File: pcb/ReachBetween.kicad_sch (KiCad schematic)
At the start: 7 parts, among them J1 USB_C_Receptacle_USB2.0, J2 USB_C_Receptacle_USB2.0, J3 USB_C_Receptacle_USB2.0

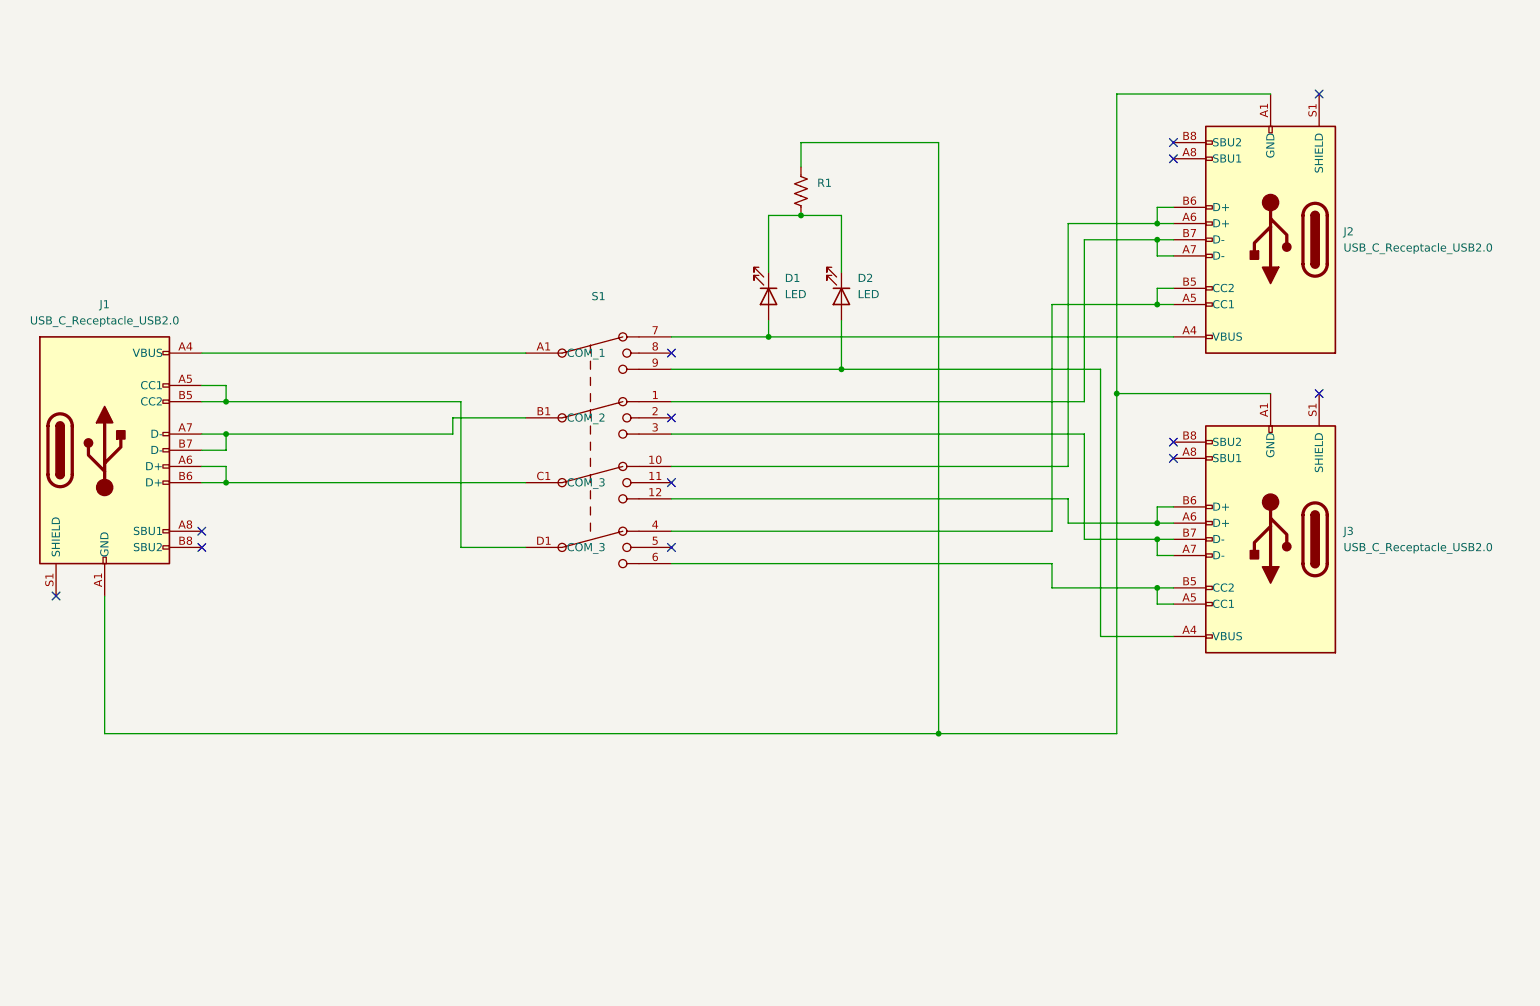
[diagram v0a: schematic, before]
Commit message: Finish board
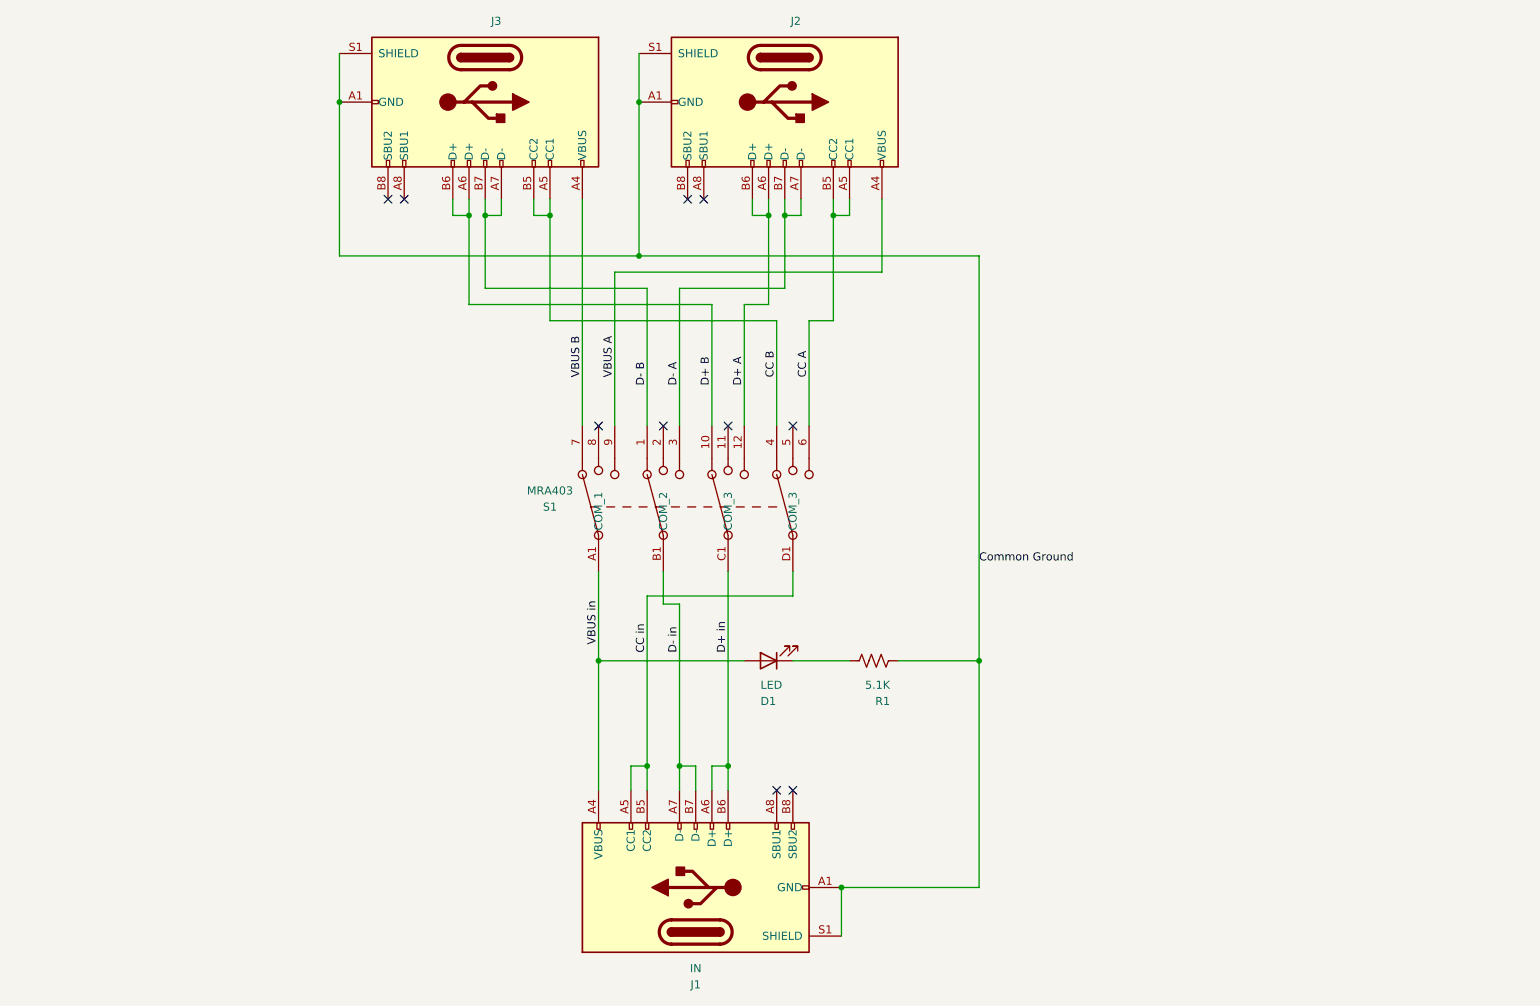
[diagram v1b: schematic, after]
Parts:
- removed D2: LED, LED_THT:LED_D5.0mm_Clear, symbol Device:LED
- J1: value USB_C_Receptacle_USB2.0 -> IN; footprint Connector_USB:USB_C_Receptacle_JAE_DX07S016JA1R1500 -> Library:USB_C_Receptacle_JAE_DX07S016JA1R1500_AislerCompatible
- J2: renamed from J3; value USB_C_Receptacle_USB2.0 -> (none); footprint Connector_USB:USB_C_Receptacle_JAE_DX07S016JA1R1500 -> Library:USB_C_Receptacle_JAE_DX07S016JA1R1500_AislerCompatible
- J3: renamed from J2; value USB_C_Receptacle_USB2.0 -> (none); footprint Connector_USB:USB_C_Receptacle_JAE_DX07S016JA1R1500 -> Library:USB_C_Receptacle_JAE_DX07S016JA1R1500_AislerCompatible
- R1: value (none) -> 5.1K
- S1: value (none) -> MRA403
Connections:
- net at D1.1 (K): now also R1.1; no longer R1.2
- net VBUS B: now reaches J3.A4 (VBUS), J3.A9 (VBUS), J3.B4 (VBUS), J3.B9 (VBUS), S1.7
- net VBUS B: no longer D1.2 (A)
- net D- B: now reaches J3.A7 (D-), J3.B7 (D-), S1.1
- net D+ B: now reaches J3.A6 (D+), J3.B6 (D+), S1.10
- net D+ A: now reaches J2.A6 (D+), J2.B6 (D+), S1.12
- net D- A: now reaches J2.A7 (D-), J2.B7 (D-), S1.3
- net CC B: now reaches J3.A5 (CC1), J3.B5 (CC2), S1.4
- net CC A: now reaches J2.A5 (CC1), J2.B5 (CC2), S1.6
- net VBUS A: now reaches J2.A4 (VBUS), J2.A9 (VBUS), J2.B4 (VBUS), J2.B9 (VBUS), S1.9
- net VBUS in: now reaches J1.A4 (VBUS), J1.A9 (VBUS), J1.B4 (VBUS), J1.B9 (VBUS), S1.A1 (COM_1)
- net VBUS in: now also D1.2 (A)
- net D- in: now reaches J1.A7 (D-), J1.B7 (D-), S1.B1 (COM_2)
- net D+ in: now reaches J1.A6 (D+), J1.B6 (D+), S1.C1 (COM_3)
- net CC in: now reaches J1.A5 (CC1), J1.B5 (CC2), S1.D1 (COM_3)
- net Common Ground: now reaches J1.A1 (GND), J1.A12 (GND), J1.B1 (GND), J1.B12 (GND), J2.A1 (GND), J2.A12 (GND), J2.B1 (GND), J2.B12 (GND), J3.A1 (GND), J3.A12 (GND), J3.B1 (GND), J3.B12 (GND)
- net Common Ground: now also J1.S1 (SHIELD), J2.S1 (SHIELD), J3.S1 (SHIELD), R1.2; no longer R1.1
- no-connect marks 13 -> 10
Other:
- moved on the sheet: D1, J1, J2, J3, R1, S1
